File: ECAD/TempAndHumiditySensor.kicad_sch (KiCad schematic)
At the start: 2 parts, among them U10 DHT11

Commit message: BOM fixed, ready to order
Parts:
- R13: Manufacturer (none) -> UNI-ROYAL(Uniroyal Elec); Manufacturer Number (none) -> 0603WAF1002T5E
- U10: Manufacturer (none) -> Aosong (Guangzhou) Elec; Manufacturer Number (none) -> DHT11
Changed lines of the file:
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@@
       (effects (font (size 1.27 1.27)) hide)
     )
-    (property "Datasheet" "~" (id 3) (at 158.75 85.09 0)
+    (property "Datasheet" "https://datasheet.lcsc.com/lcsc/1811062009_UNI-ROYAL-Uniroyal-Elec-0603WAF1002T5E_C25804.pdf" (id 3) (at 158.75 85.09 0)
+      (effects (font (size 1.27 1.27)) hide)
+    )
+    (property "Manufacturer" "UNI-ROYAL(Uniroyal Elec)" (id 4) (at 158.75 85.09 0)
+      (effects (font (size 1.27 1.27)) hide)
+    )
+    (property "Manufacturer Number" "0603WAF1002T5E" (id 5) (at 158.75 85.09 0)
       (effects (font (size 1.27 1.27)) hide)
     )
@@
       (effects (font (size 1.27 1.27)) hide)
     )
+    (property "Manufacturer" "Aosong (Guangzhou) Elec" (id 4) (at 144.78 92.71 0)
+      (effects (font (size 1.27 1.27)) hide)
+    )
+    (property "Manufacturer Number" "DHT11" (id 5) (at 144.78 92.71 0)
+      (effects (font (size 1.27 1.27)) hide)
+    )

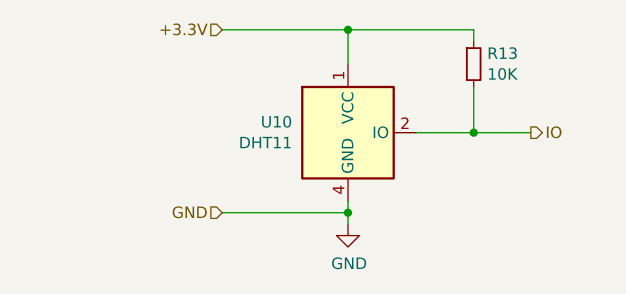
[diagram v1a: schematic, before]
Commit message: adding production and step files
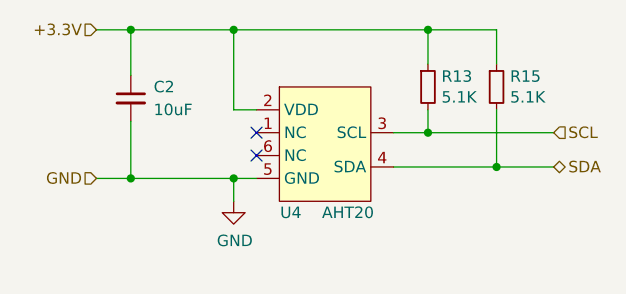
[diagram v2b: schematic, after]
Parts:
- removed U10: DHT11, Sensor:Aosong_DHT11_5.5x12.0_P2.54mm, symbol Sensor:DHT11
- added C2: 10uF, Capacitor_SMD:C_0603_1608Metric, symbol Device:C_Small
- added R15: 5.1K, Resistor_SMD:R_0603_1608Metric, symbol Device:R_Small
- added U4: AHT20, Package_DFN:SOIC-6, symbol User_Sensors:AHT20
- R13: value 10K -> 5.1K; Manufacturer UNI-ROYAL(Uniroyal Elec) -> UNI-ROYAL(Uniroyal Elec); Manufacturer Number 0603WAF1002T5E -> 0603WAF5101T5E; Package (none) -> 0603
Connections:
- net +3.3V: now also C2.1, R15.1, U4.2 (VDD)
- net GND: now also C2.2, U4.5 (GND)
- net IO renamed SCL
- net SCL: now also U4.3 (SCL)
- new net SDA: R15.2, U4.4 (SDA)
- no-connect marks 0 -> 2
